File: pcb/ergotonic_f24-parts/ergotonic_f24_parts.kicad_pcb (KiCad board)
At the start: 2 copper layers, 117.1 x 149 mm, 12 parts

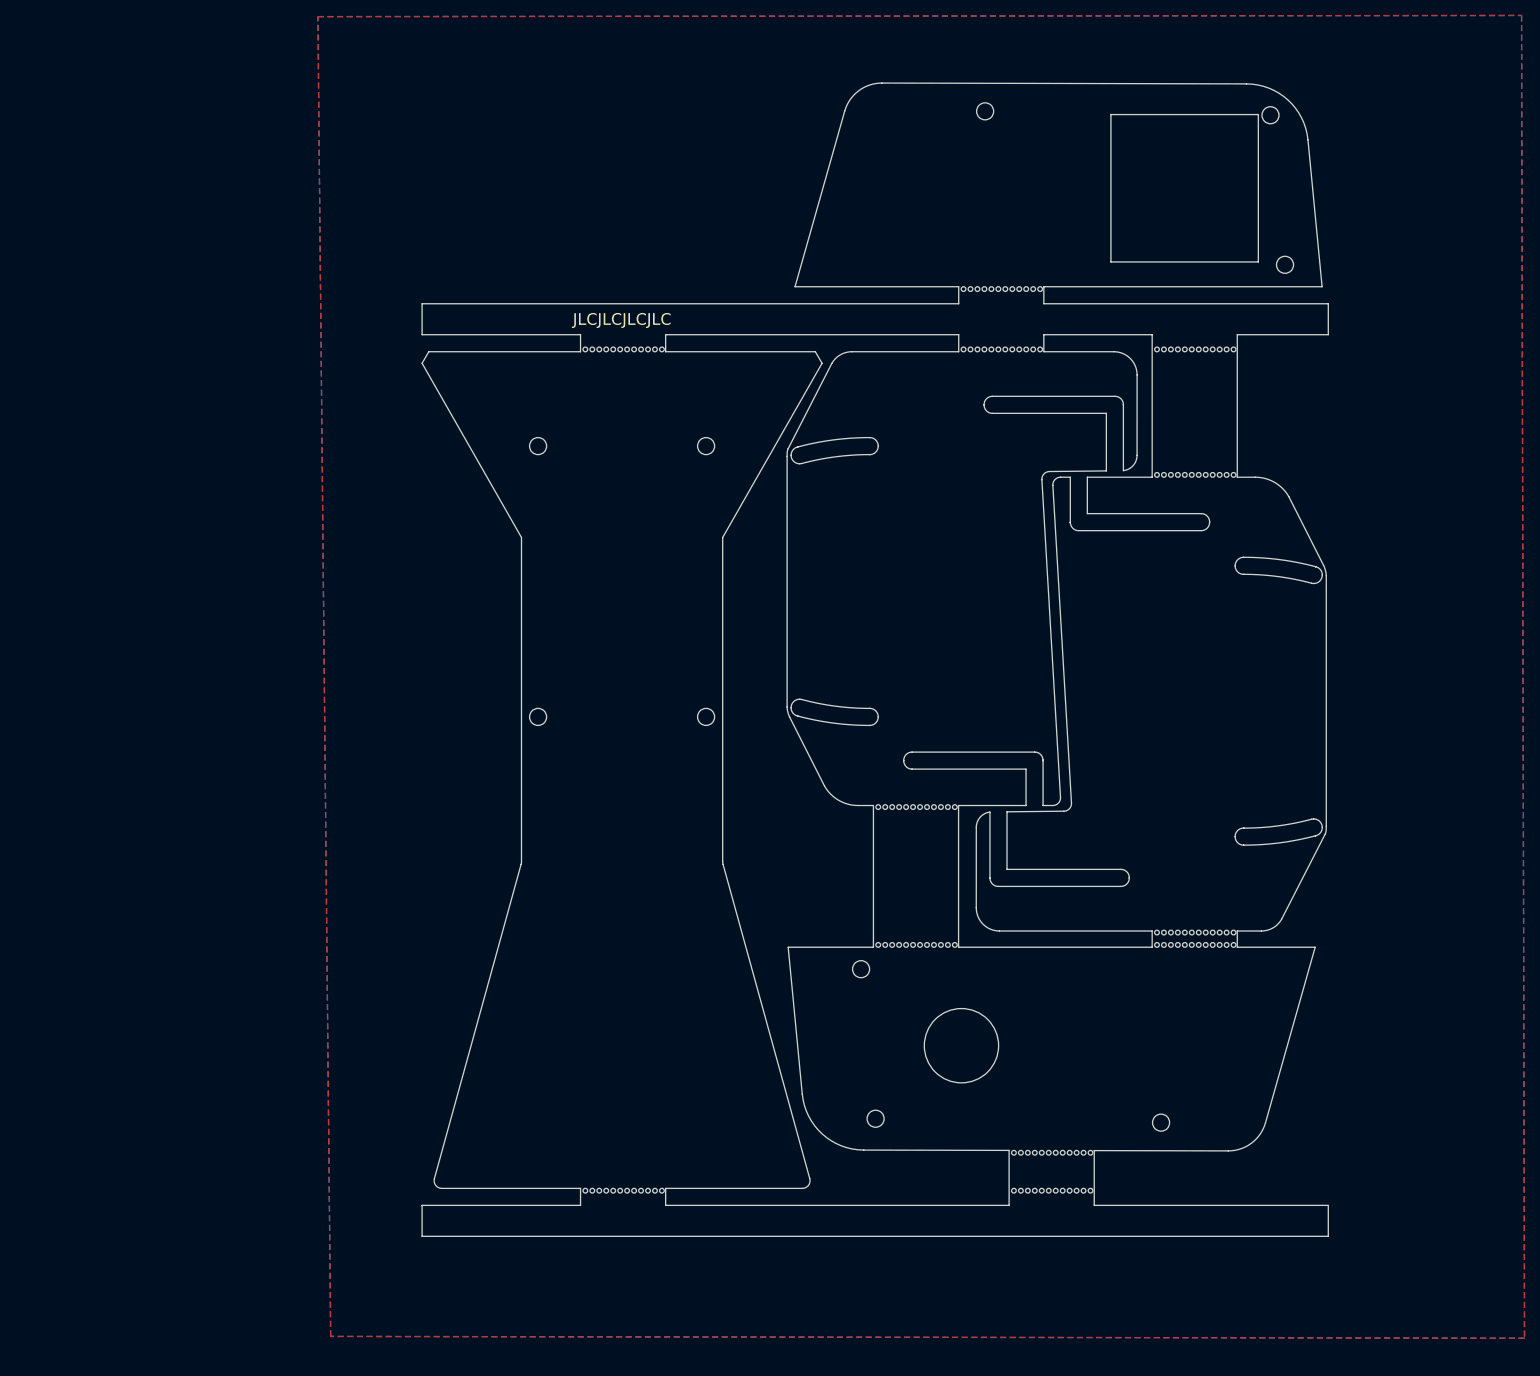
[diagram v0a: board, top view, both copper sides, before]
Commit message: Version 1 Revision 3
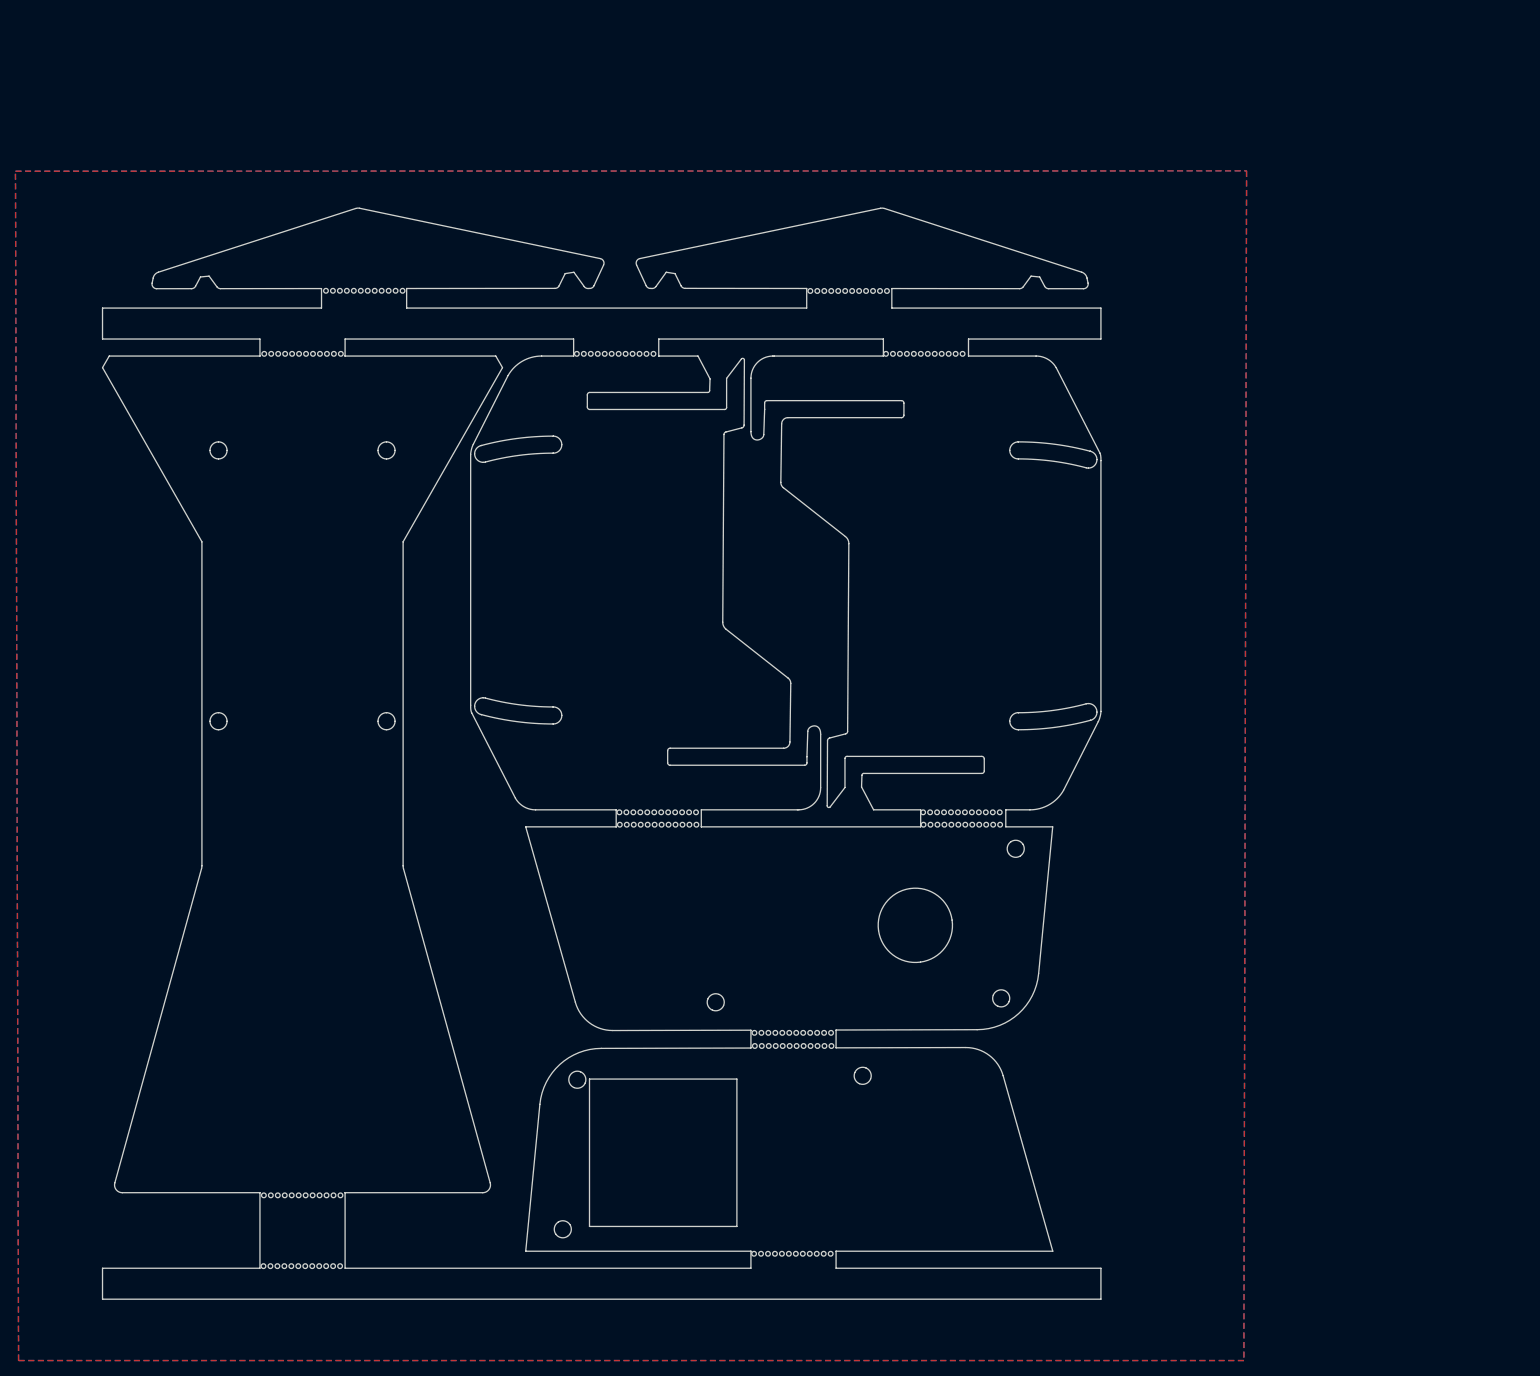
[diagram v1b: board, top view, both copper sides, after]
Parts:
- added mb27: mousebite, e3w2q:mousebite, F.Cu at (-68.0, -1.07)
- added mb27: mousebite, e3w2q:mousebite, F.Cu at (-130.6, -1.10)
- moved mb1 97.5 mm to (-138.7, 125.0)
- moved mb2 97.1 mm to (-138.6, 115.8)
- moved mb20 92.7 mm to (-92.6, 67.9)
- moved mb19 82.0 mm to (-92.7, 66.3)
- moved mb11 53.6 mm to (-75.2, 96.5)
- moved mb30 50.7 mm to (-98.2, 7.05)
- moved mb27 41.5 mm to (-138.6, 7.05)
- moved mb12 33.2 mm to (-53.4, 67.9)
- moved mb8 23.3 mm to (-75.2, 123.3)
- moved mb15 19.6 mm to (-75.2, 94.8)
- moved mb29 10.0 mm to (-58.2, 7.05)
- moved mb16 5.84 mm to (-53.4, 66.3)
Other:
- board size 117.1 x 149 mm -> 129 x 141 mm
- board text removed: "JLCJLCJLCJLC"
